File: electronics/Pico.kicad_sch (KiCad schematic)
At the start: 36 parts, among them J1 USB_B_Micro, J7 Conn_ARM_JTAG_SWD_10, J9 Conn_01x08, SW1 PTS645SK50SMTR92LFS, U1 STM32F415RGTx, U4 USBLC6-2SC6, Y2 Crystal_GND24

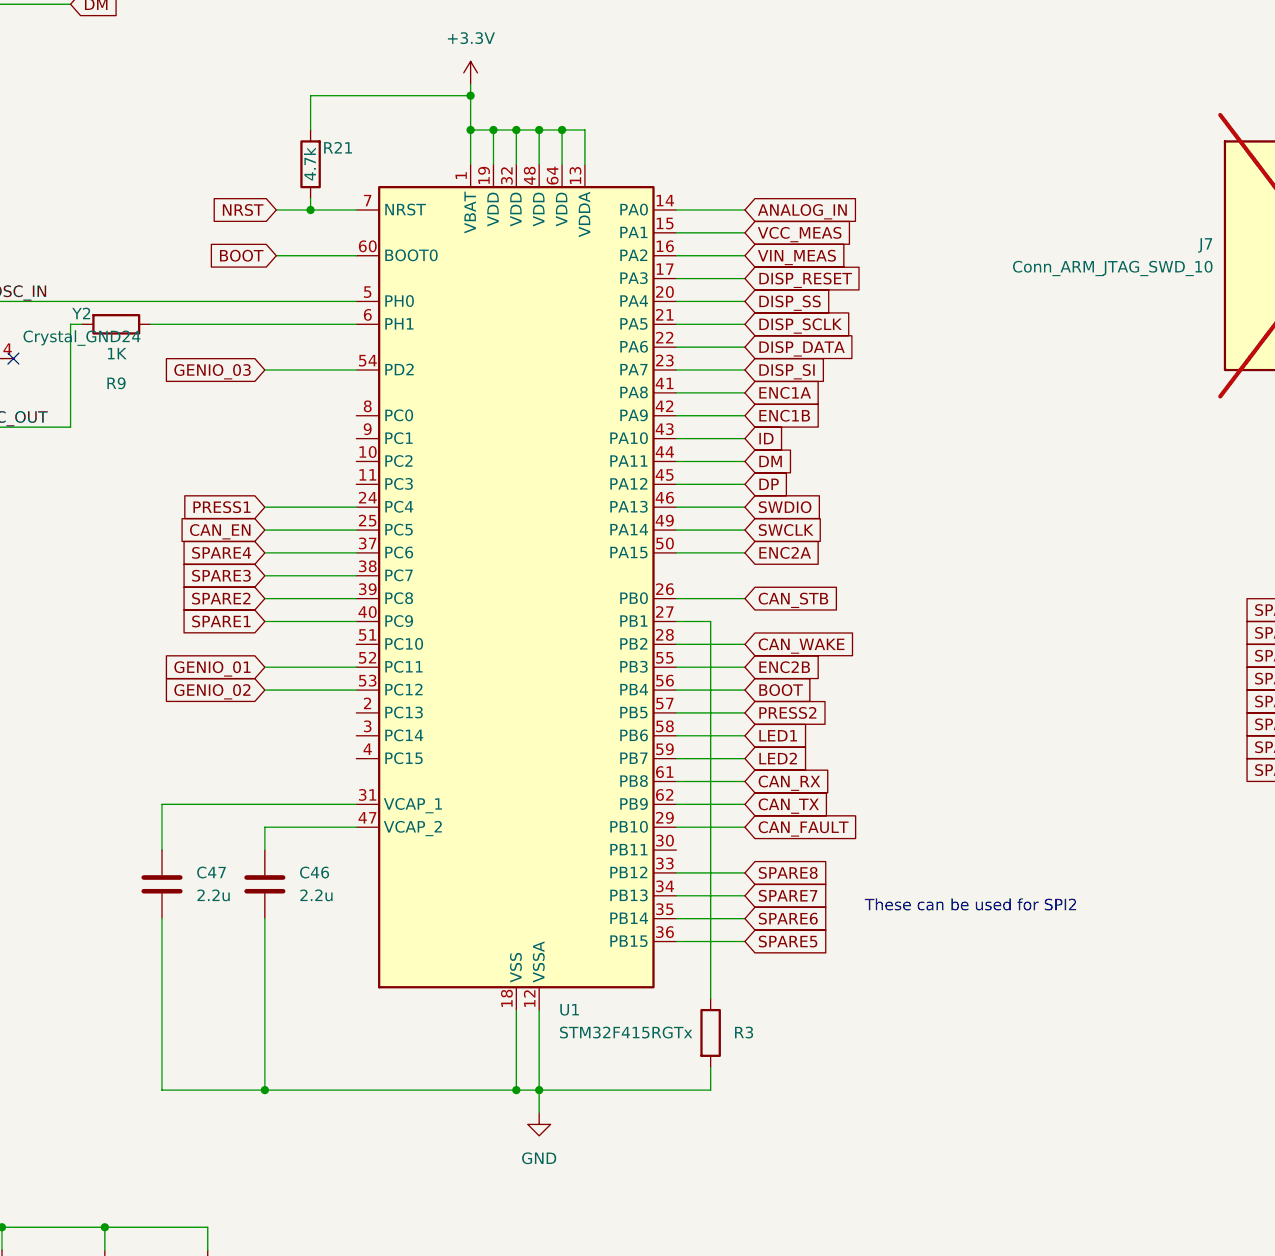
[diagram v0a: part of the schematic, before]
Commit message: Updated design for REV B.
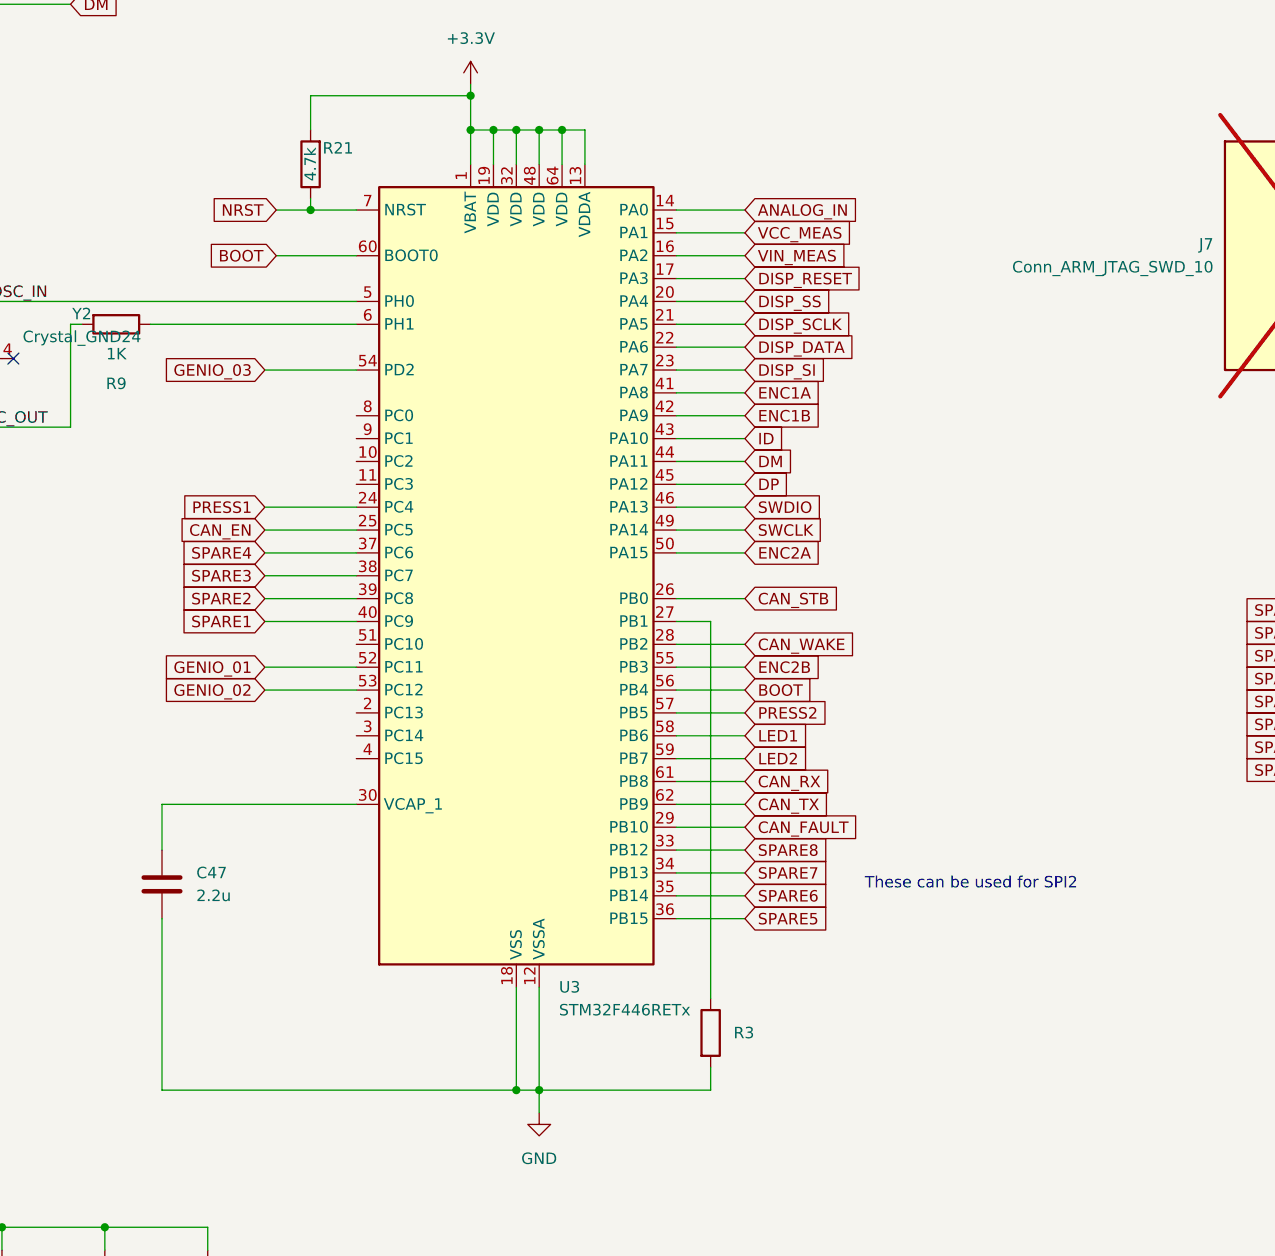
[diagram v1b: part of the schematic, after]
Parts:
- removed C46: 2.2u, Capacitor_SMD:C_0603_1608Metric, symbol Device:C
- removed U1: STM32F415RGTx, Package_QFP:LQFP-64_10x10mm_P0.5mm, symbol MCU_ST_STM32F4:STM32F415RGTx
- added U3: STM32F446RETx, Package_QFP:LQFP-64_10x10mm_P0.5mm, symbol MCU_ST_STM32F4:STM32F446RETx
- R2, R3: JLCPCB (none) -> C102750
- R21: JLCPCB (none) -> C103059
- R5, R6: JLCPCB (none) -> C25152
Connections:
- net +3.3V: now also U3.1 (VBAT), U3.13 (VDDA), U3.19 (VDD), U3.32 (VDD), U3.48 (VDD), U3.64 (VDD)
- net ANALOG_IN: now also U3.14 (PA0)
- net BOOT: now also U3.56 (PB4), U3.60 (BOOT0)
- net CAN_EN: now also U3.25 (PC5)
- net CAN_FAULT: now also U3.29 (PB10)
- net CAN_RX: now also U3.61 (PB8)
- net CAN_STB: now also U3.26 (PB0)
- net CAN_TX: now also U3.62 (PB9)
- net CAN_WAKE: now also U3.28 (PB2)
- net DISP_DATA: now also U3.22 (PA6)
- net DISP_RESET: now also U3.17 (PA3)
- net DISP_SCLK: now also U3.21 (PA5)
- net DISP_SI: now also U3.23 (PA7)
- net DISP_SS: now also U3.20 (PA4)
- net DM: now also U3.44 (PA11)
- net DP: now also U3.45 (PA12)
- net ENC1A: now also U3.41 (PA8)
- net ENC1B: now also U3.42 (PA9)
- net ENC2A: now also U3.50 (PA15)
- net ENC2B: now also U3.55 (PB3)
- net GENIO_01: now also U3.52 (PC11)
- net GENIO_02: now also U3.53 (PC12)
- net GENIO_03: now also U3.54 (PD2)
- net GND: now also U3.12 (VSSA), U3.18 (VSS), U3.31 (VSS), U3.47 (VSS), U3.63 (VSS)
- net ID: now also U3.43 (PA10)
- net LED1: now also U3.58 (PB6)
- net LED2: now also U3.59 (PB7)
- net NRST: now also U3.7 (NRST)
- net OSC_IN: now also U3.5 (PH0)
- net PRESS1: now also U3.24 (PC4)
- net PRESS2: now also U3.57 (PB5)
- net SPARE1: now also U3.40 (PC9)
- net SPARE2: now also U3.39 (PC8)
- net SPARE3: now also U3.38 (PC7)
- net SPARE4: now also U3.37 (PC6)
- net SPARE5: now also U3.36 (PB15)
- net SPARE6: now also U3.35 (PB14)
- net SPARE7: now also U3.34 (PB13)
- net SPARE8: now also U3.33 (PB12)
- net SWCLK: now also U3.49 (PA14)
- net SWDIO: now also U3.46 (PA13)
- net VCC_MEAS: now also U3.15 (PA1)
- net VIN_MEAS: now also U3.16 (PA2)
- net at R9.1: now also U3.6 (PH1)
- net at R3.1: now also U3.27 (PB1)
- net at C47.1: now also U3.30 (VCAP_1)

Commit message: This version is working well. Need to figure out USB DFU programming.
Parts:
- C1: JLCPCB (none) -> C1779
- R1: footprint Resistor_SMD:R_0603_1608Metric -> Resistor_SMD:R_0402_1005Metric; JLCPCB (none) -> C25126
- R4, R9: JLCPCB (none) -> C11702
- R7, R8: JLCPCB (none) -> C12246
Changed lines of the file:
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@@
+			)
+		)
+		(property "JLCPCB" "C12246"
+			(at 256.54 22.86 0)
+			(effects
+				(font
+					(size 1.27 1.27)
+				)
+				(hide yes)
 			)
 		)
@@
 			)
 		)
-		(property "Footprint" "Resistor_SMD:R_0603_1608Metric"
+		(property "Footprint" "Resistor_SMD:R_0402_1005Metric"
 			(at 36.068 48.26 90)
 			(effects
@@
 			)
 		)
-		(property "JLCPCB" ""
+		(property "JLCPCB" "C25126"
 			(at 34.29 48.26 0)
 			(effects
@@
 		)
 		(property "Description" ""
+			(at 256.54 31.75 0)
+			(effects
+				(font
+					(size 1.27 1.27)
+				)
+				(hide yes)
+			)
+		)
+		(property "JLCPCB" "C12246"
 			(at 256.54 31.75 0)
 			(effects
@@
 			)
 		)
-		(property "JLCPCB" ""
+		(property "JLCPCB" "C11702"
 			(at 107.95 74.93 0)
 			(effects
@@
 			)
 		)
-		(property "JLCPCB" ""
+		(property "JLCPCB" "C1779"
 			(at 19.05 181.61 0)
 			(effects
@@
 			)
 		)
-		(property "JLCPCB" ""
+		(property "JLCPCB" "C11702"
 			(at 67.31 113.03 0)
 			(effects
